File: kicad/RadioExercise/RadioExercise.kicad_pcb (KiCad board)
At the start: 2 copper layers, 50 x 40 mm, 17 parts, among them IC1 HT82V739, IC2 PIC16F1778-I_SP, IC3 SST26VF064B-104I_SM, J1 Conn_01x02_Female, SW1 SW_Push, SW2 SW_Push, SW5 SW_DPDT_x2

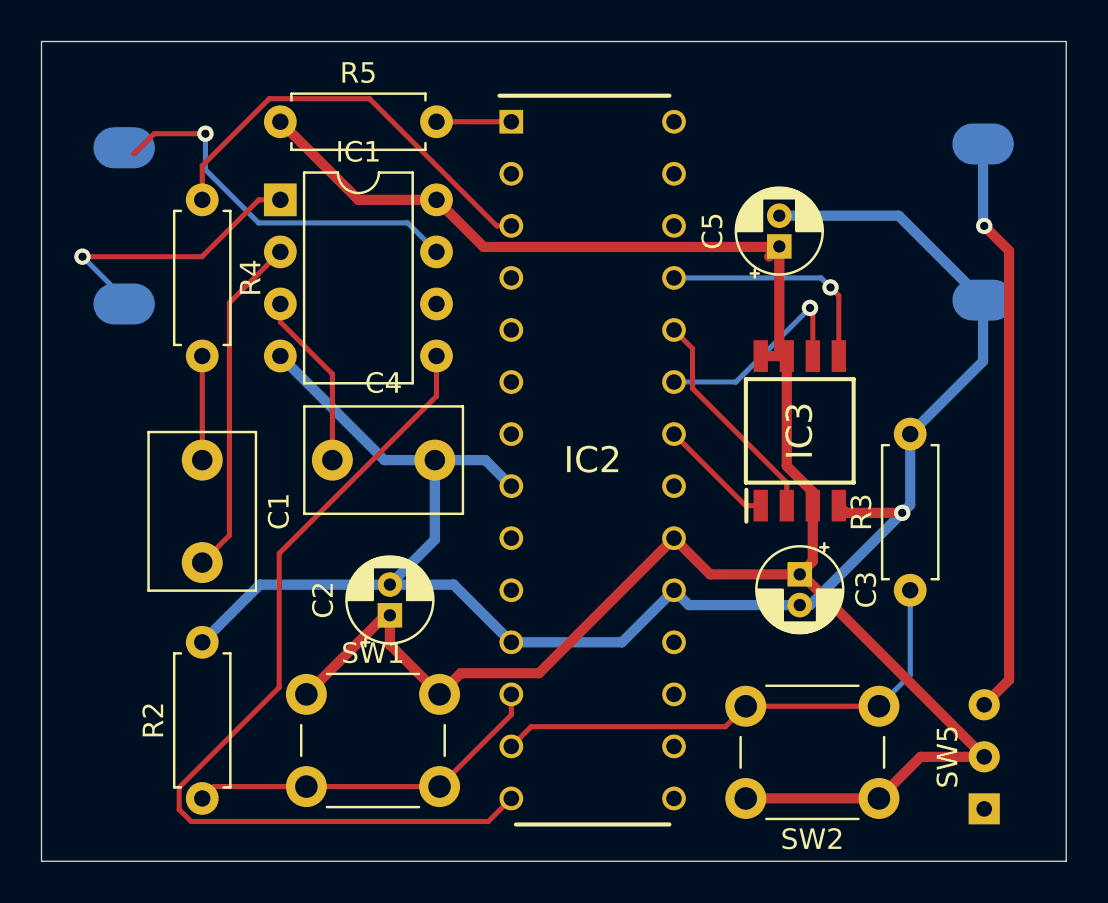
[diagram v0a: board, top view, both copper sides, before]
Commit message: update
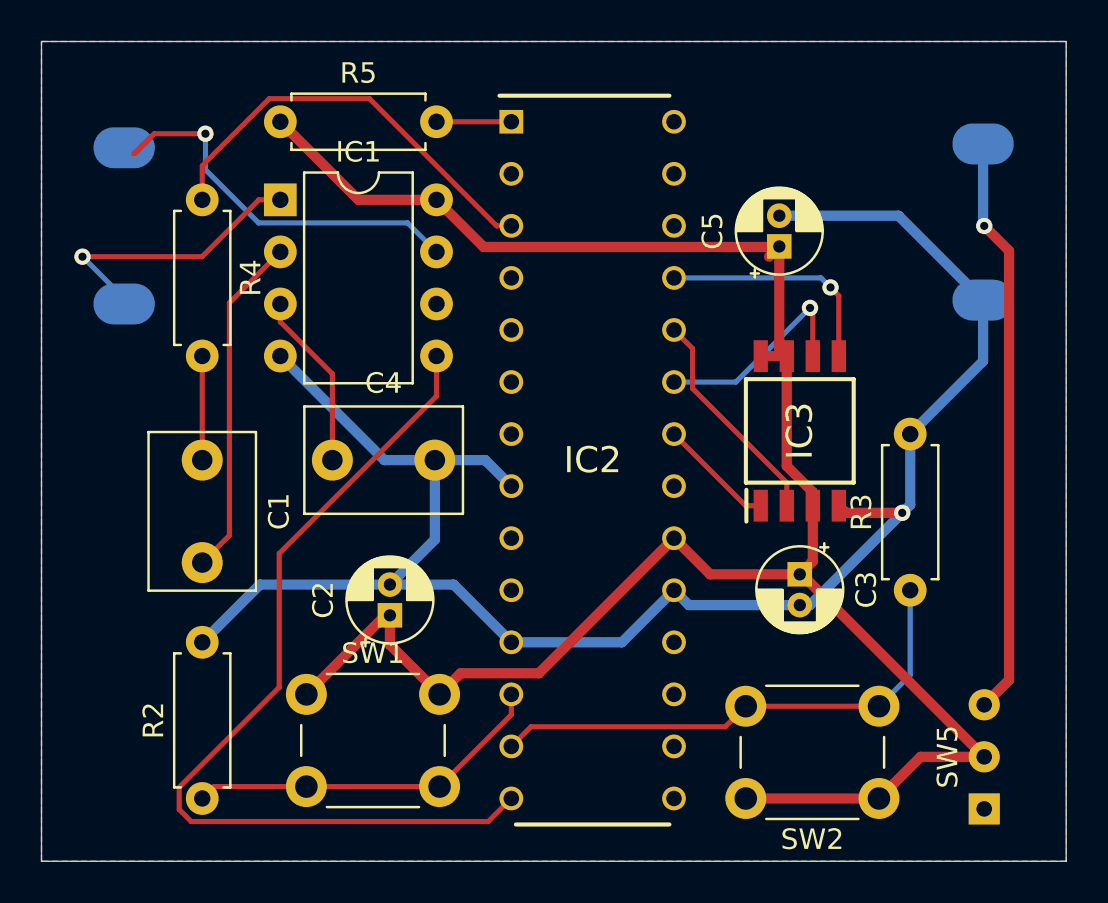
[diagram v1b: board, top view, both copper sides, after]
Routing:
- added copper zone on B.Cu, net GND
- added copper zone on F.Cu, net VDD
